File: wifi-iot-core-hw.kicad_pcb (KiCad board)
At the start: 2 copper layers, 34.3 x 61 mm, 49 parts, among them P1 USB, P10 CONN_01X01, P11 CONN_01X01, P3 CONN_01X16, P4 CONN_01X04, P5 CONN_01X16, P6 CONN_01X03, P7 CONN_01X03, P8 CONN_01X01, P9 CONN_01X01, U1 LP2985LV, U2 STM32F103C8Tx, U3 ESP-07v2, Y1 8MHz

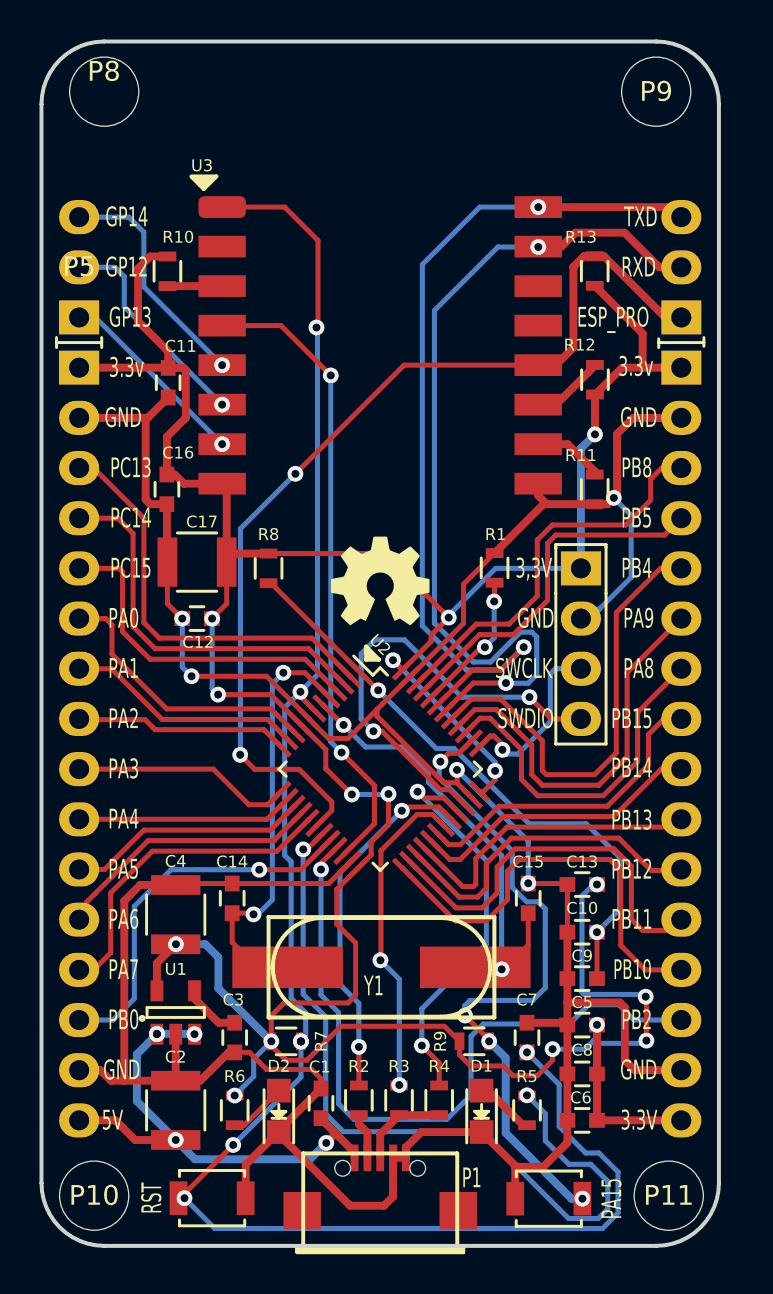
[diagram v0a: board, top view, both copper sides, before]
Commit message: Fix Schematic & PCB
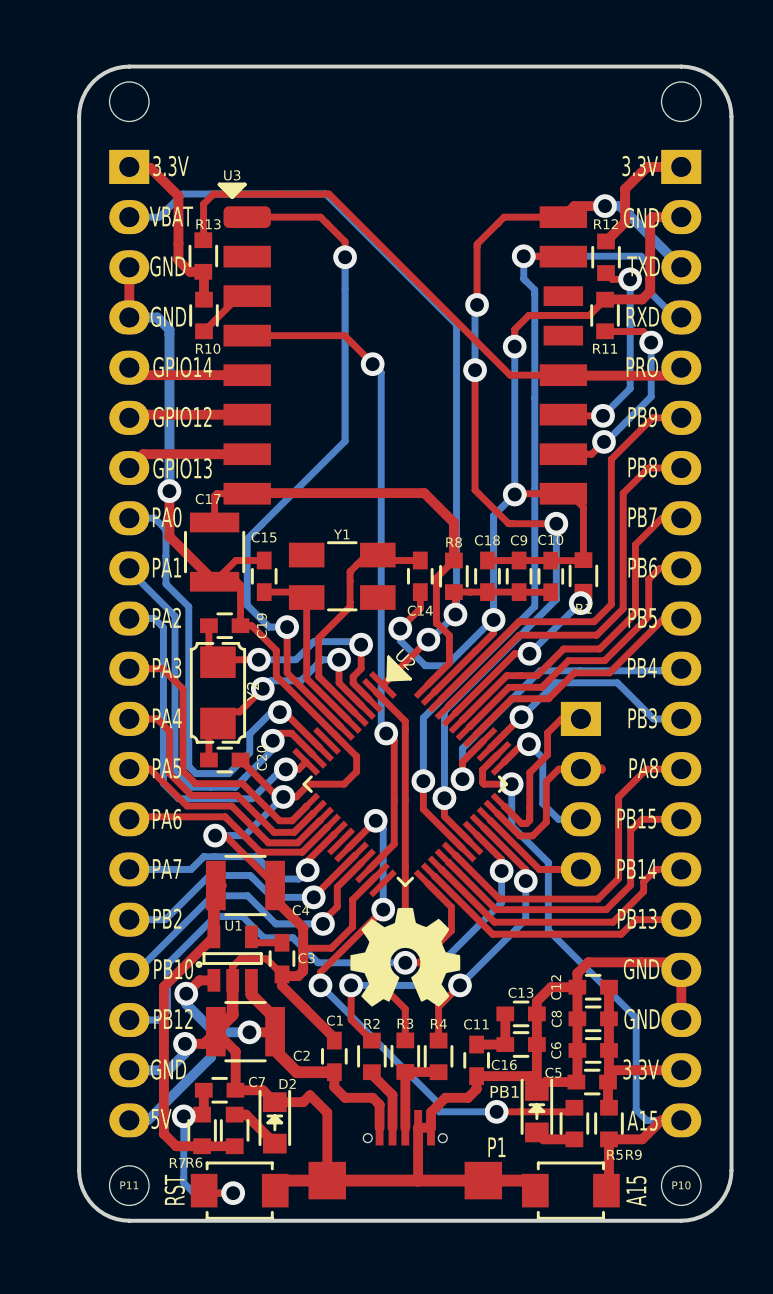
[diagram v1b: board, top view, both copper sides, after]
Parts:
- removed D1: Led PWR, LEDs:LED_0805
- removed G***: logo5_silkscreen-front_5mm, logo:logo5_silkscreen-front_5mm
- removed P5: CONN_01X16, Pin_Headers:Pin_Header_Straight_1x16
- removed P6, P7: CONN_01X03, Pin_Headers:Pin_Header_Straight_1x03
- removed PA15: SW_PUSH_SMALL_H, Buttons_Switches_SMD:SW_SPST_B3U-1000P-B
- removed the RST at (113.4, 133.5)
- added A15: SW_PUSH_SMALL_H, lib:SW_SPST_B3U-1000P-B, F.Cu at (131.6, 133.1)
- added C18: 100nF, lib:C_0603, F.Cu at (127.3, 102.0)
- added C19: 15pF, lib:C_0603, F.Cu at (114.0, 104.5)
- added C20: 15pf, lib:C_0603, F.Cu at (114.0, 111.3)
- added P2: CONN_01X20, Pin_Headers:Pin_Header_Straight_1x20, F.Cu at (109.2, 81.3)
- added PB1: Led PWR, LEDs:LED_0805, F.Cu at (129.8, 129.1)
- added RST: RST, lib:SW_SPST_B3U-1000P-B, F.Cu at (114.8, 133.1)
- added VAL**: oshw_logo_500, lib:logo5, F.Cu at (123.2, 121.3)
- added Y2: 32.687, lib:crystal_smd_32.768_2Pin, F.Cu at (113.7, 107.9)
- C1, C10, C11, C12, C13, C14, C15, C16, C5, C6, C7, C8, C9: footprint Capacitors_SMD:C_0603 -> lib:C_0603
- C3: value 1uF -> 10nF; footprint Capacitors_SMD:C_0603 -> lib:C_0603
- P1: footprint w_conn_pc:conn_usb_B_micro_smd-2 -> lib:Micro_usb_B_smd
- P10, P11, P8, P9: footprint Mounting_Holes:MountingHole_3.5mm -> lib:MountingHole_2mm
- P3: value CONN_01X16 -> CONN_01X20; footprint Pin_Headers:Pin_Header_Straight_1x16 -> Pin_Headers:Pin_Header_Straight_1x20
- R1, R10, R11, R12, R13, R2, R3, R4, R5, R6, R7, R8, R9: footprint Resistors_SMD:R_0603 -> lib:R_0603
- U2: footprint Housings_QFP:LQFP-48_7x7mm_Pitch0.5mm -> lib:LQFP-48_Pin1.7x0.3mm_Pitch0.5mm
- U3: footprint ESP8266:ESP-07v2-smd-16pin -> lib:ESP-07v2-smd-16pin
- Y1: footprint Crystal:HC49_sm -> lib:Crystal_SMD_5032_4Pads
- moved C11 37.7 mm to (126.8, 126.5)
- moved C16 33.3 mm to (129.1, 125.7), turned to 0 degrees
- moved P10 29.7 mm to (137.2, 132.8)
- moved C12 27.4 mm to (132.7, 122.8)
- moved P11 27.3 mm to (109.2, 132.8)
- moved C15 21.1 mm to (116.0, 102.0)
- moved C9 20.6 mm to (128.9, 102.0), turned to 270 degrees
- moved Y1 19.9 mm to (120.0, 102.0), turned to 180 degrees
- moved R13 19.8 mm to (113.0, 85.8)
- moved C14 18.9 mm to (124.0, 102.0), turned to 270 degrees
- moved C10 18.1 mm to (130.6, 102.0), turned to 270 degrees
- moved C7 15.8 mm to (113.8, 128.0), turned to 0 degrees
- moved P3 10.2 mm to (137.2, 81.3)
- moved R8 9.39 mm to (125.7, 102.0)
- moved R11 8.81 mm to (133.3, 88.8), turned to 90 degrees
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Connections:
- net /OSC_IN renamed Net-(C14-Pad1)
- net /OSC_OUT renamed Net-(C15-Pad1)
- P3 pad 10: PB15 -> PB5
- P3 pad 11: PB14 -> PB4
- P3 pad 12: PB13 -> PB3
- P3 pad 13: PB12 -> PA8
- P3 pad 14: PB10 -> PB15
- P3 pad 15: GNDREF -> PB14
- P3 pad 16: +3V3 -> PB13
- P3 pad 3: PB9 -> /ESP_TXD
- P3 pad 4: PB8 -> /ESP_RXD
- P3 pad 5: PB5 -> /PRO
- P3 pad 6: PB4 -> PB9
- P3 pad 7: PB3 -> PB8
- P3 pad 8: PA9 -> PB7
- P3 pad 9: PA8 -> PB6
- R13 pad 2: ESP_PRO -> /PRO
- U2 pad 18: ESP_PRO -> /PRO
- U2 pad 2: PA13 -> /USB_DIS
- U2 pad 3: PA14 -> Net-(C19-Pad1)
- U2 pad 30: PA9 -> /ESP_RXD
- U2 pad 31: /USB_DIS -> /ESP_TXD
- U2 pad 4: PA15 -> Net-(C20-Pad1)
- U2 pad 42: RXD -> PB6
- U2 pad 43: TXD -> PB7
- U3 pad 12: ESP_PRO -> /PRO
- U3 pad 15: RXD -> /ESP_RXD
- U3 pad 16: TXD -> /ESP_TXD
- U3 pad 5: Net-(P6-Pad3) -> GPIO14
- U3 pad 6: Net-(P6-Pad2) -> GPIO12
- U3 pad 7: Net-(P6-Pad1) -> GPIO13
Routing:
- net +3V3: track 173.3 -> 80.3 mm, vias 17 -> 0
- net ESP_PRO: track 50.3 -> 0.00 mm, vias 2 -> 0
- net /NRST: track 93.4 -> 44.4 mm, vias 7 -> 4
- net /ESP_TXD: track 0.00 -> 48.7 mm, vias 0 -> 5
- net /ESP_RXD: track 0.00 -> 45.5 mm, vias 0 -> 2
- net TXD: track 44.9 -> 0.00 mm, vias 2 -> 0
- net RXD: track 44.8 -> 0.00 mm, vias 2 -> 0
- net GNDREF: track 172.4 -> 203.9 mm, vias 6 -> 8
- net /PRO: track 0.00 -> 30.2 mm
- net PA13: track 21.2 -> 0.00 mm
- net PA14: track 19.6 -> 0.00 mm
- net PB10: track 35.8 -> 16.9 mm, vias 2 -> 1
- net /SWDIO: track 23.5 -> 5.61 mm, vias 2 -> 0
- net PA15: track 17.4 -> 0.00 mm
- net PB7: track 0.00 -> 17.4 mm
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- removed copper zone on B.Cu, net GNDREF
- removed copper zone on F.Cu, net GNDREF
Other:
- board size 34.3 x 61 mm -> 33 x 58.4 mm
- net class Default: trace_width 0.4 -> 0.35; via_dia 0.8 -> 1.2; via_drill 0.4 -> 0.7
- rule trace_min: 0.25 -> 0.3
- rule via_min_drill: 0.3 -> 0.7
- rule via_min_size: 0.8 -> 1.2
- board text added: "A15"
- board text added: "GPIO12"
- board text added: "GPIO13"
- board text added: "GPIO14"
- board text added: "PB3"
- board text added: "PB6"
- board text added: "PB7"
- board text added: "PB9"
- board text added: "PRO"
- board text added: "VBAT"
- board text removed: "3,3V"
- board text removed: "3.3v"
- board text removed: "ESP_PRO"
- board text removed: "GP12"
- board text removed: "GP13"
- board text removed: "GP14"
- board text removed: "PA9"
- board text removed: "PB0"
- board text removed: "PB11"
- board text removed: "PC13"
- board text removed: "PC14"
- board text removed: "PC15"
- board text removed: "SWCLK"
- board text removed: "SWDIO"
